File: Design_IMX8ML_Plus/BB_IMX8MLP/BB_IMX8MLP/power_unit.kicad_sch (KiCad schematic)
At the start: 65 parts, among them J10 Barrel_Jack, Q1 PMDT290UCE, Q2 NTMFS5C670NLT1G, Q3 NTMFS5C670NLT1G, Q4 PMDT290UCE, SW1 Power ON/OFF, SW2 RESET, SW3 RECOVERY, U4 LTC4368IDD-1_PBF, U5 AOZ2261AQI-15, U6 NCV4274CST50T3G, U7 AOZ2261AQI-15, U8 LTC2954CDDB-1-TRMPBF

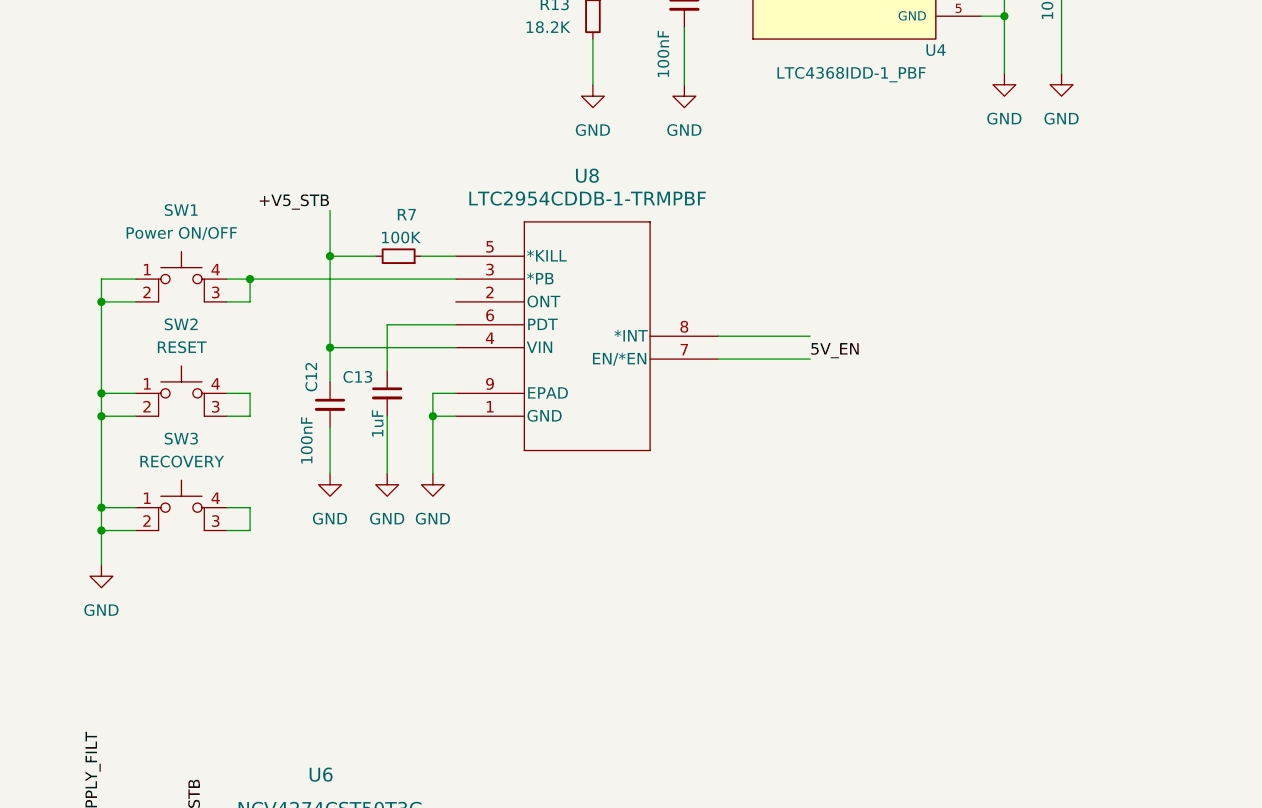
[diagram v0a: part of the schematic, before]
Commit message: improving the usb conector
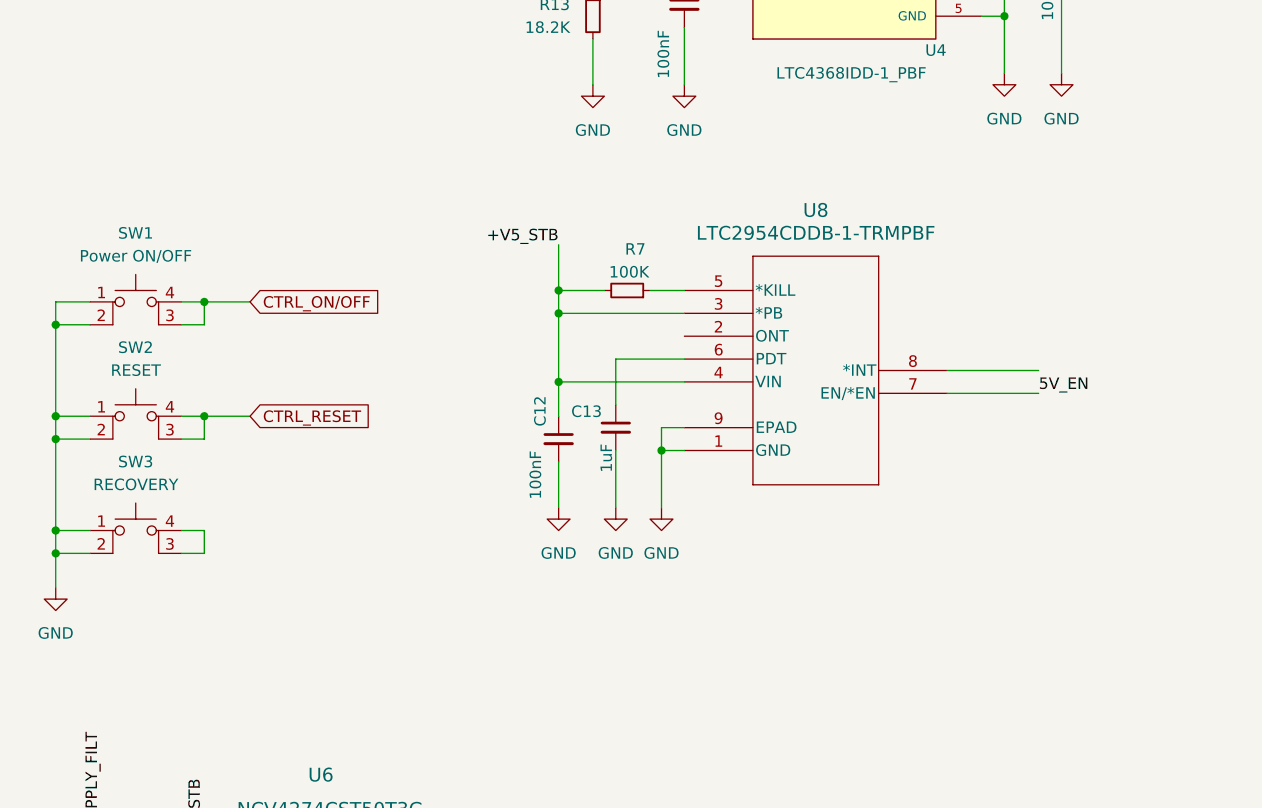
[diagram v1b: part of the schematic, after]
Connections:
- net +V5_STB: now also U8.3 (*PB)
- net CTRL_ON/OFF: now reaches SW1.3 (K), SW1.4 (A)
- net CTRL_ON/OFF: no longer U8.3 (*PB)
- net CTRL_RESET: now reaches SW2.3 (K), SW2.4 (A)
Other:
- moved on the sheet: C12, C13, R7, SW1, SW2, SW3, U8
